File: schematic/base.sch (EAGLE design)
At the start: 11 parts, among them IC1 MEGA328-PU

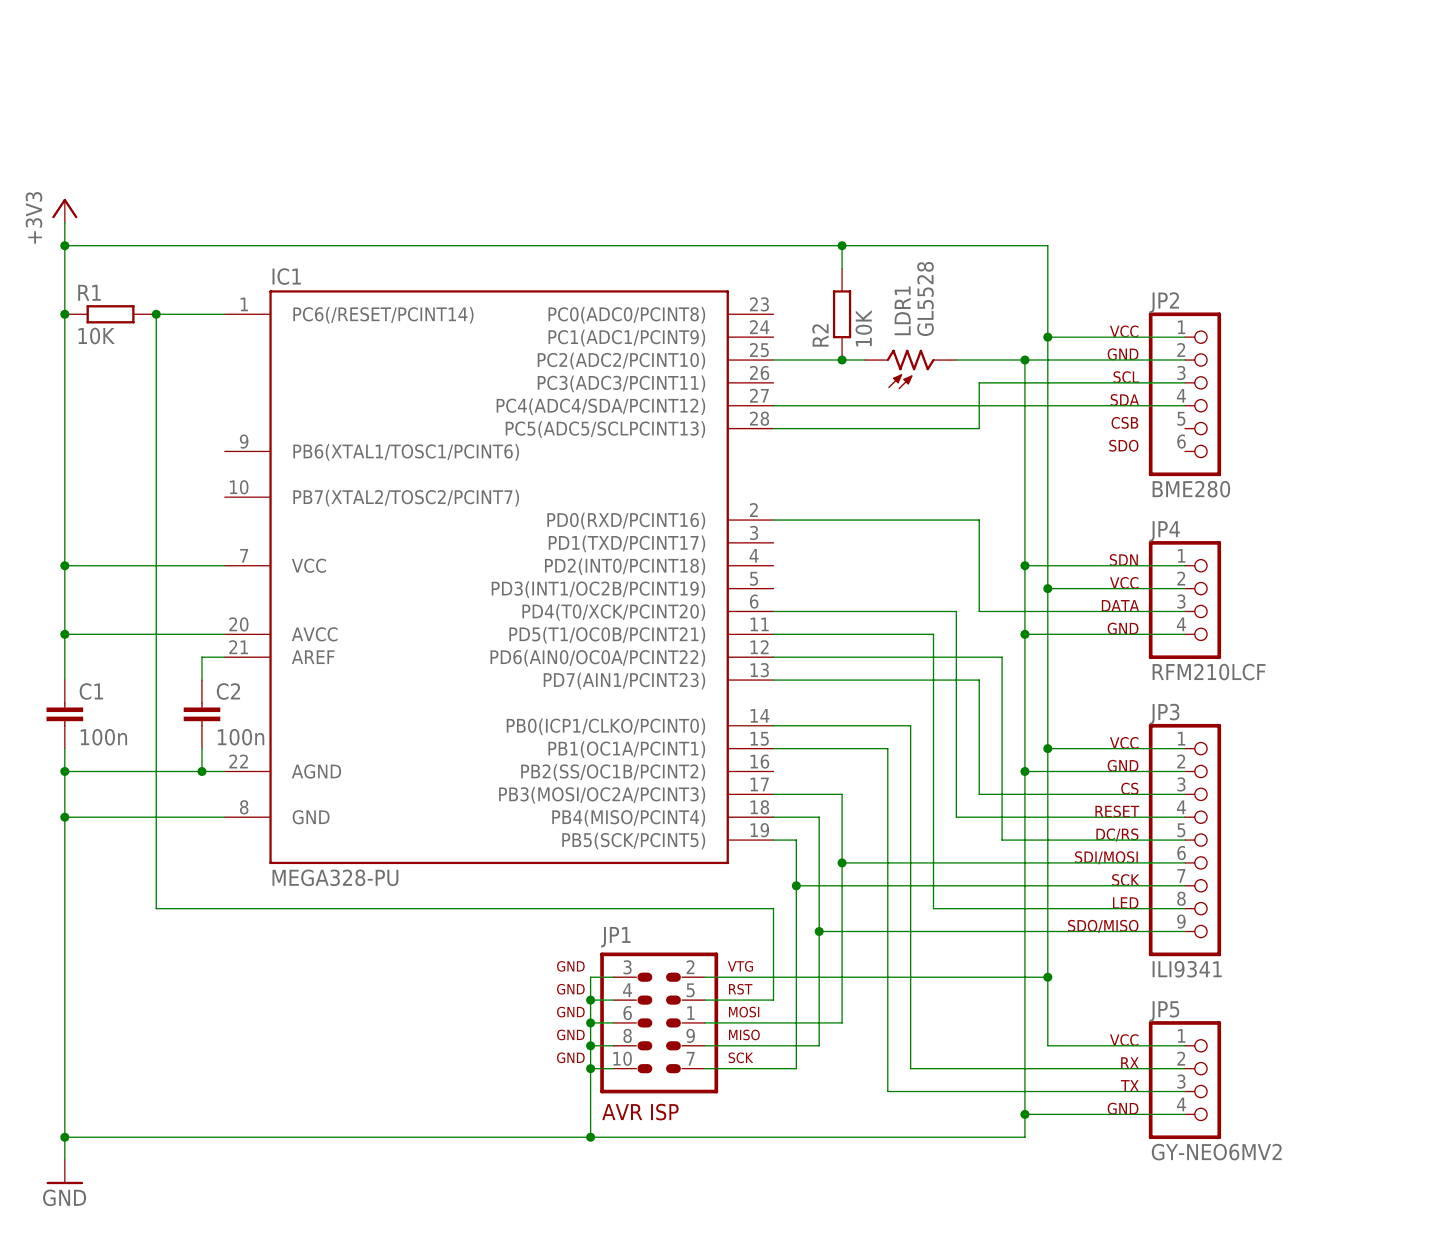
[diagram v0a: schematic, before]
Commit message: Add files via upload
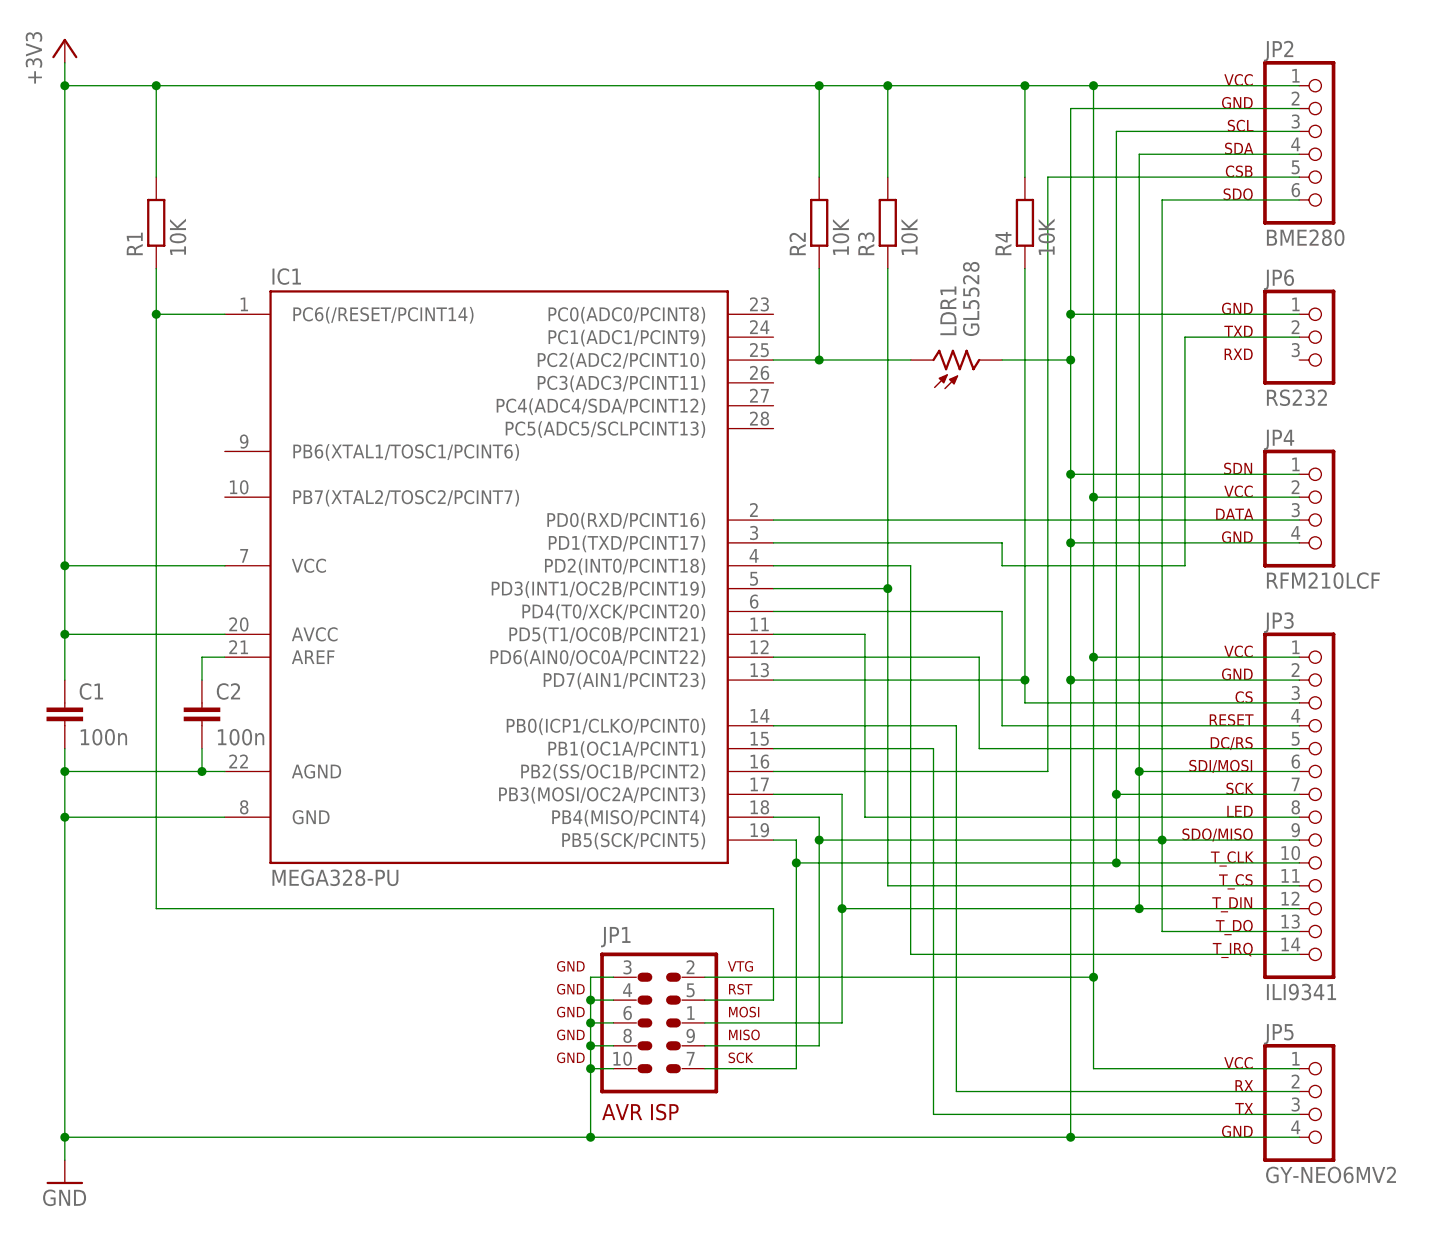
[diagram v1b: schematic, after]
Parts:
- added JP6: RS232, pinhead:PINHD-1X3
- added R3, R4: 10K, rcl:R-EU_0204/7
- JP3: device pinhead:PINHD-1X9 -> pinhead:PINHD-1X14
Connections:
- new net N$16: IC1.PD3(INT1/OC2B/PCINT19), JP3.11, R3.1
- new net N$17: IC1.PD1(TXD/PCINT17), JP6.2
- net +3V3: now also R1.2, R3.2, R4.2; no longer R1.1
- net GND: now also JP6.1
- net N$1: now also IC1.PB2(SS/OC1B/PCINT2), JP2.5; no longer IC1.PC4(ADC4/SDA/PCINT12), JP2.4
- net N$12: now also JP2.3, JP3.10
- net N$2: now also R1.1; no longer R1.2
- net N$3: now also IC1.PB4(MISO/PCINT4), JP1.9, JP2.6, JP3.13, JP3.9; no longer IC1.PC5(ADC5/SCLPCINT13), JP2.3
- net N$7: now also R4.1
- net N$8: now also JP2.4, JP3.12
- net N$9: now also IC1.PD2(INT0/PCINT18), JP3.14; no longer IC1.PB4(MISO/PCINT4), JP1.9, JP3.9
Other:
- note added: "GND TXD RXD"
- note added: "VCC GND CS RESET DC/RS SDI/MOSI SCK LED SDO/MISO T_CLK T_CS T_DIN T_DO T_IRQ"
- note removed: "VCC GND CS RESET DC/RS SDI/MOSI SCK LED SDO/MISO"
- moved on the sheet: JP2, JP4, JP5, LDR1, R1, R2
